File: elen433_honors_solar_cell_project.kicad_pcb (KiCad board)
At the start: 2 copper layers, 33 x 53 mm, 6 parts, among them J1 Conn_01x02

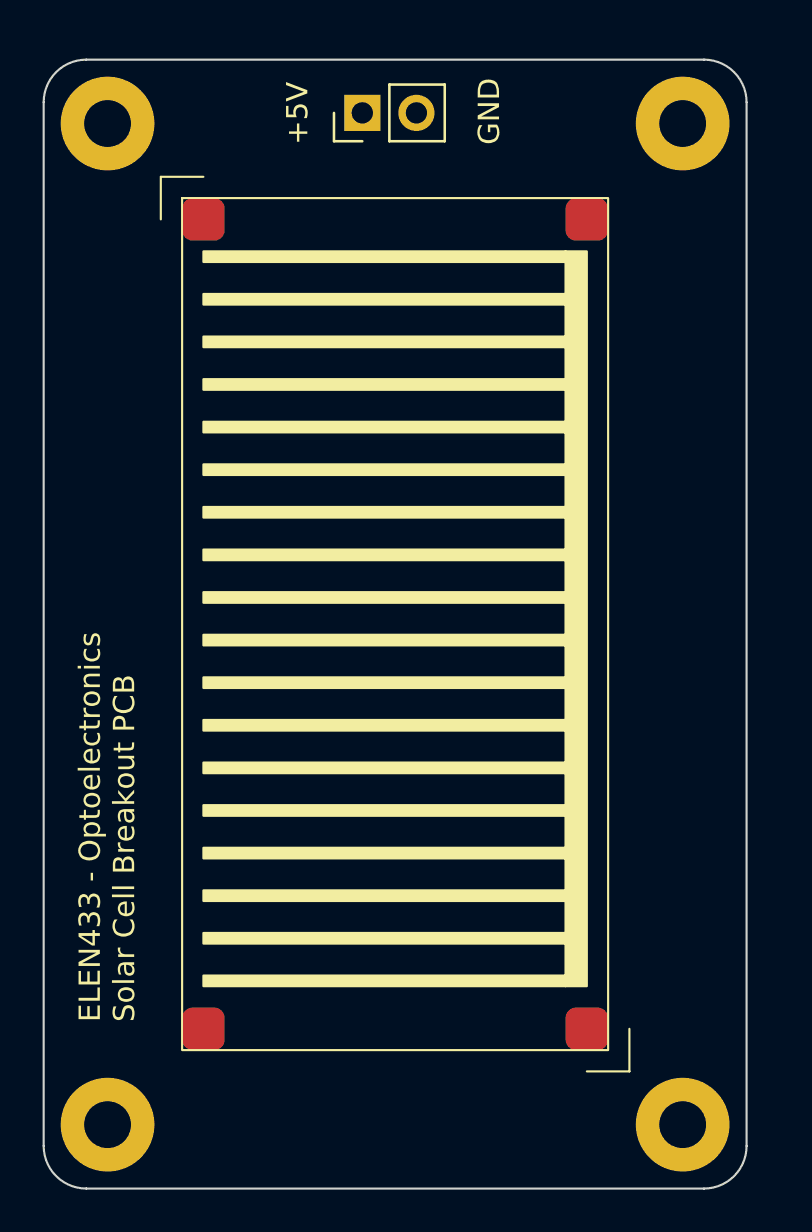
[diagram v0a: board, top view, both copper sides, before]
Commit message: Created board
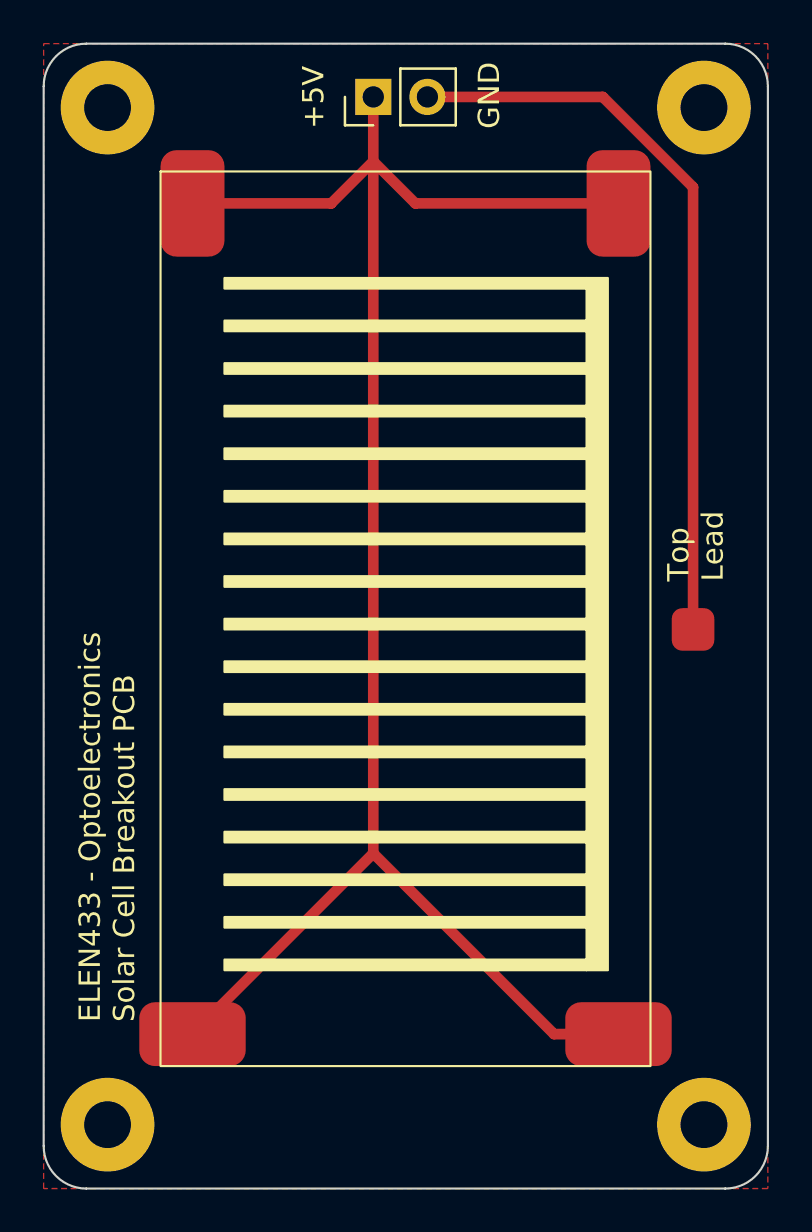
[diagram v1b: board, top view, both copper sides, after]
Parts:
- moved H1 1.25 mm to (157.5, 50.8)
- moved U1 1.02 mm to (134.0, 95.2)
- moved H3 1.00 mm to (157.5, 98.5)
- moved J1 0.91 mm to (142.0, 50.2)
- moved H2 0.75 mm to (129.5, 50.8)
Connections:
- U1 pad 1: (no net) -> +5V
- U1 pad 2: (no net) -> GND
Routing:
- net +5V: track 0.00 -> 84.2 mm
- net GND: track 0.00 -> 35.7 mm
- added copper zone on F.Cu, net GND
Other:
- board size 33 x 53 mm -> 34 x 53.8 mm
- board text added: "Top Lead"
